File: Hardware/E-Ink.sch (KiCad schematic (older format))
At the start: 34 parts

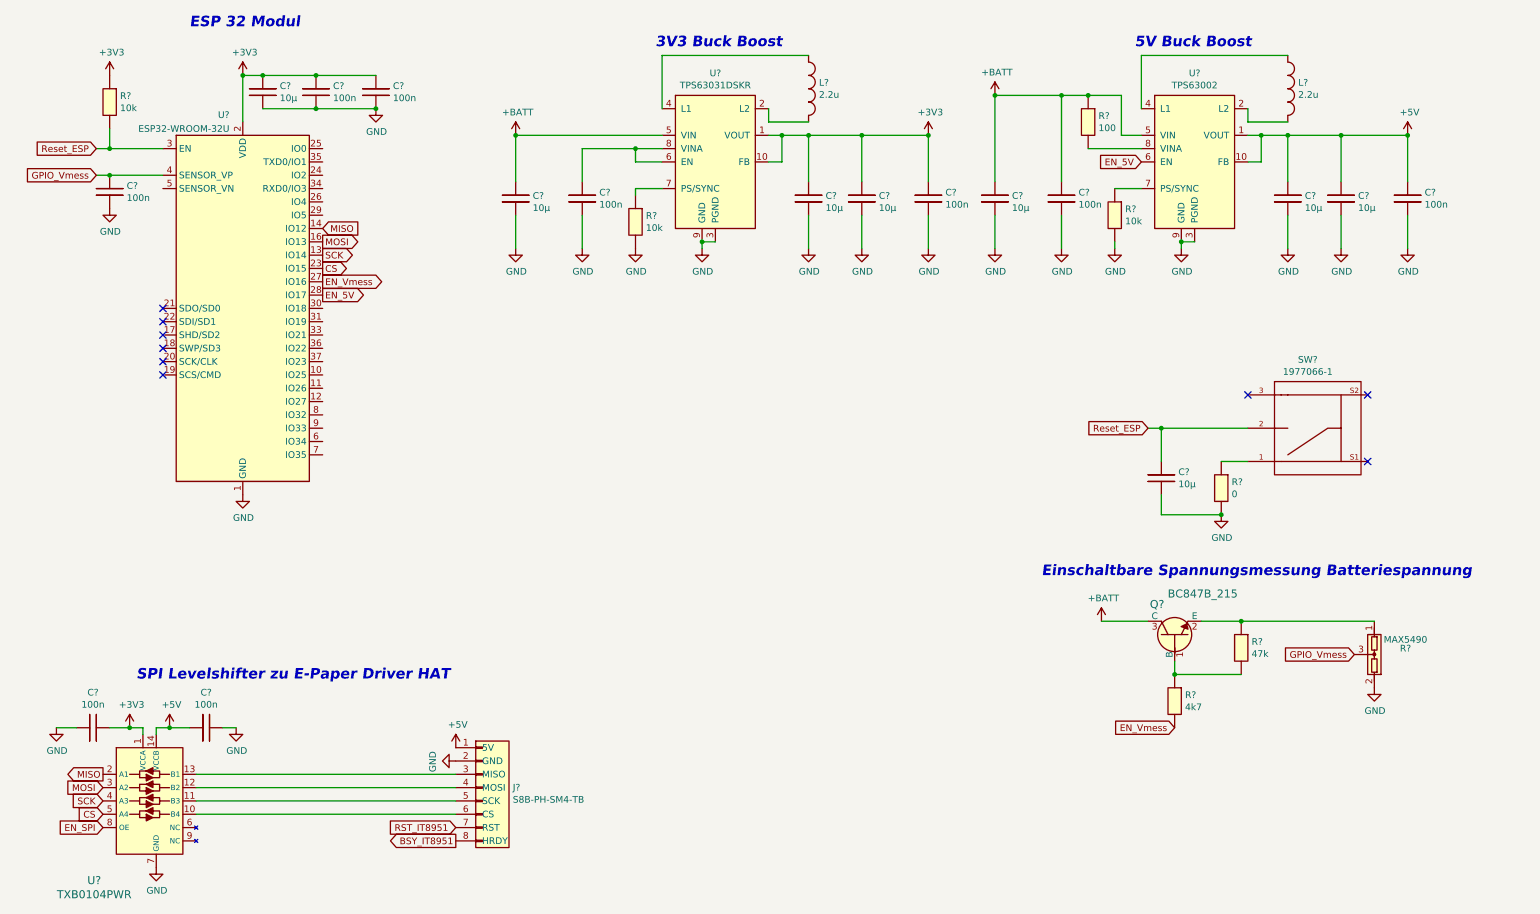
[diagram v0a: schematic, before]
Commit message: Save work at OTH
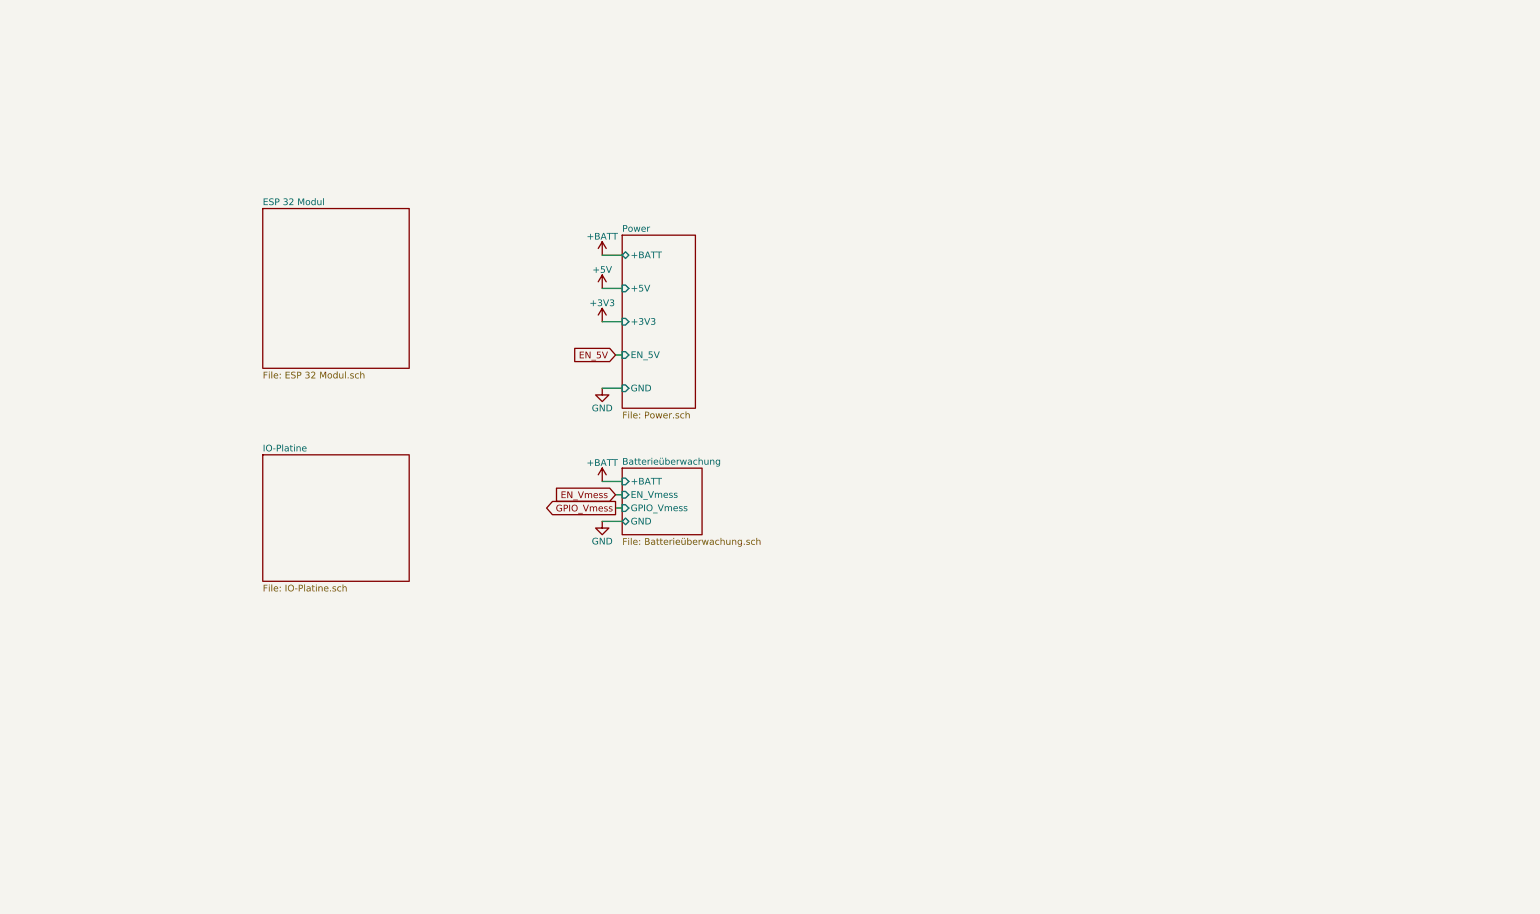
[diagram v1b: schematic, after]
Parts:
- removed C? (x9): 100n, Capacitor_SMD:C_0805_2012Metric_Pad1.15x1.40mm_HandSolder, symbol E-Ink:100n
- removed C? (x8): 10µ, Capacitor_SMD:C_0805_2012Metric_Pad1.15x1.40mm_HandSolder, symbol E-Ink:10µ
- removed J?: S8B-PH-SM4-TB, symbol E-Ink:S8B-PH-SM4-TB
- removed L? (x2): 2.2u, symbol E-Ink:2.2u
- removed Q?: BC847B_215, digikey-footprints:SOT-23-3, symbol dk_Transistors-Bipolar-BJT-Single:BC847B_215
- removed R?: MAX5490, Package_TO_SOT_SMD:SOT-23, symbol E-Ink:MAX5490
- removed R?: 47k, Resistor_SMD:R_0805_2012Metric_Pad1.15x1.40mm_HandSolder, symbol E-Ink:47k
- removed R?: 4k7, Resistor_SMD:R_0805_2012Metric_Pad1.15x1.40mm_HandSolder, symbol E-Ink:4k7
- removed R? (x3): 10k, Resistor_SMD:R_0805_2012Metric_Pad1.15x1.40mm_HandSolder, symbol E-Ink:10k
- removed R?: 100, Resistor_SMD:R_0805_2012Metric_Pad1.15x1.40mm_HandSolder, symbol E-Ink:100
- removed R?: 0, Resistor_SMD:R_0805_2012Metric_Pad1.15x1.40mm_HandSolder, symbol E-Ink:0
- removed SW?: 1977066-1, TE_1977066-1, symbol Pavel_privat:1977066-1
- removed U?: ESP32-WROOM-32U, RF_Module:ESP32-WROOM-32U, symbol E-Ink:ESP32-WROOM-32U
- removed U?: TXB0104PWR, digikey-footprints:TSSOP-14_W4.4mm, symbol E-Ink:TXB0104PWR
- removed U?: TPS63031DSKR, Package_SON:Texas_S-PWSON-N10, symbol E-Ink:TPS63031DSKR
- removed U?: TPS63002, Package_SON:Texas_DRC0010J_ThermalVias, symbol E-Ink:TPS63002DRCR
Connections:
- no-connect marks 9 -> 0
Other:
- note removed: "3V3 Buck Boost"
- note removed: "5V Buck Boost"
- note removed: "ESP 32 Modul\n"
- note removed: "Einschaltbare Spannungsmessung Batteriespannung\n\n"
- note removed: "SPI Levelshifter zu E-Paper Driver HAT\n"

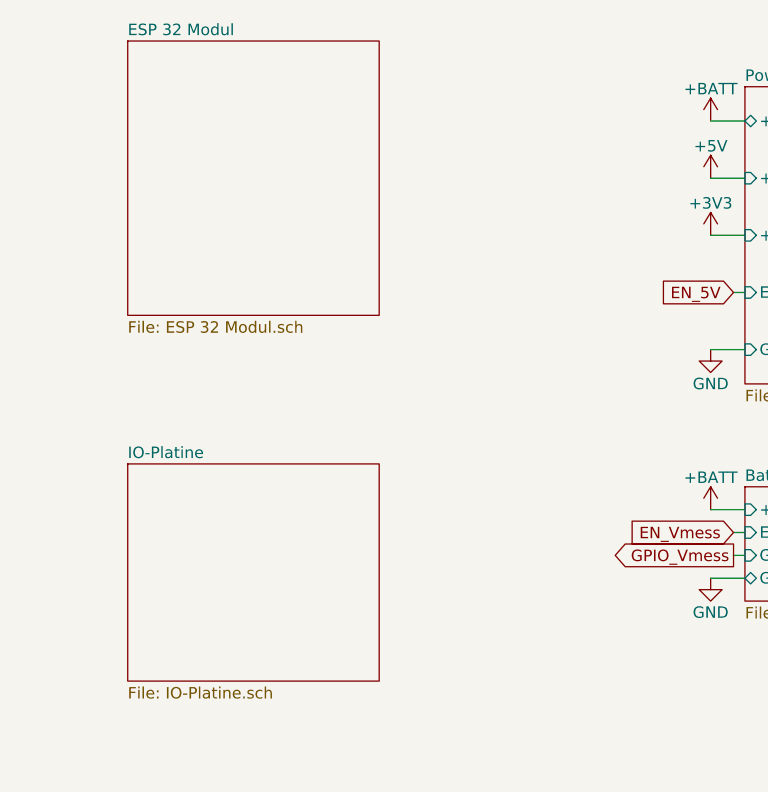
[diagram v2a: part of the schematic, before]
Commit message: Save work from OTH
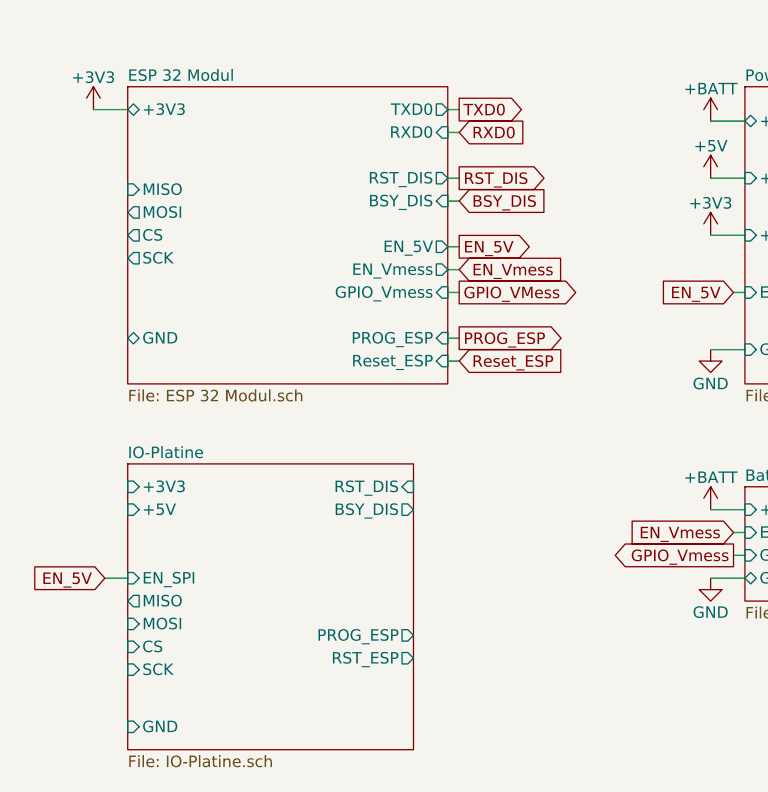
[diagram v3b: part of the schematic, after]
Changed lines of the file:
@@
 EESchema Schematic File Version 4
-EELAYER 30 0
+LIBS:E-Ink-cache
+EELAYER 29 0
 EELAYER END
 $Descr A4 11693 8268
@@
 	4900 4550 4950 4550
 $Sheet
-S 2250 2300 1100 1200
+S 2250 2500 1400 1300
 U 5DE5A7F7
 F0 "ESP 32 Modul" 50
 F1 "ESP 32 Modul.sch" 50
-$EndSheet
-$Sheet
-S 2250 4150 1100 950
-U 5DE7403E
-F0 "IO-Platine" 50
-F1 "IO-Platine.sch" 50
+F2 "Reset_ESP" I R 3650 3700 50
+F3 "GPIO_Vmess" I R 3650 3400 50
+F4 "GND" B L 2250 3600 50
+F5 "+3V3" B L 2250 2600 50
+F6 "TXD0" O R 3650 2600 50
+F7 "MISO" I L 2250 2950 50
+F8 "RXD0" I R 3650 2700 50
+F9 "EN_5V" O R 3650 3200 50
+F10 "EN_Vmess" O R 3650 3300 50
+F11 "CS" O L 2250 3150 50
+F12 "SCK" O L 2250 3250 50
+F13 "MOSI" O L 2250 3050 50
+F14 "PROG_ESP" I R 3650 3600 50
+F15 "RST_DIS" O R 3650 2900 50
+F16 "BSY_DIS" I R 3650 3000 50
 $EndSheet
 $Comp
@@
 Wire Wire Line
 	4800 4650 4950 4650
+$Sheet
+S 2250 4150 1250 1250
+U 5DE7403E
+F0 "IO-Platine" 50
+F1 "IO-Platine.sch" 50
+F2 "EN_SPI" I L 2250 4650 50
+F3 "CS" I L 2250 4950 50
+F4 "SCK" I L 2250 5050 50
+F5 "MOSI" I L 2250 4850 50
+F6 "MISO" O L 2250 4750 50
+F7 "RST_ESP" O R 3500 5000 50
+F8 "+3V3" I L 2250 4250 50
+F9 "+5V" I L 2250 4350 50
+F10 "GND" I L 2250 5300 50
+F11 "RST_DIS" I R 3500 4250 50
+F12 "BSY_DIS" O R 3500 4350 50
+F13 "PROG_ESP" O R 3500 4900 50
+$EndSheet
+$Comp
+L power:+3V3 #PWR?
+U 1 1 5DE68EE7
+P 2100 2600
+F 0 "#PWR?" H 2100 2450 50  0001 C CNN
+F 1 "+3V3" H 2100 2740 50  0000 C CNN
+F 2 "" H 2100 2600 50  0001 C CNN
+F 3 "" H 2100 2600 50  0001 C CNN
+	1    2100 2600
+	1    0    0    -1
+$EndComp
+Wire Wire Line
+	2100 2600 2250 2600
+Text GLabel 3700 2600 2    50   Output ~ 0
+TXD0
+Text GLabel 3700 2700 2    50   Input ~ 0
+RXD0
+Wire Wire Line
+	3700 2600 3650 2600
+Wire Wire Line
+	3650 2700 3700 2700
+Text GLabel 3700 2900 2    50   Output ~ 0
+RST_DIS
+Text GLabel 3700 3000 2    50   Input ~ 0
+BSY_DIS
+Wire Wire Line
+	3700 2900 3650 2900
+Wire Wire Line
+	3650 3000 3700 3000
+Text GLabel 3700 3200 2    50   Output ~ 0
+EN_5V
+Text GLabel 3700 3300 2    50   Input ~ 0
+EN_Vmess
+Wire Wire Line
+	3700 3200 3650 3200
+Wire Wire Line
+	3650 3300 3700 3300
+Text GLabel 3700 3400 2    50   Output ~ 0
+GPIO_VMess
+Wire Wire Line
+	3700 3400 3650 3400
+Text GLabel 3700 3600 2    50   Output ~ 0
+PROG_ESP
+Text GLabel 3700 3700 2    50   Input ~ 0
+Reset_ESP
+Wire Wire Line
+	3700 3600 3650 3600
+Wire Wire Line
+	3650 3700 3700 3700
+Text GLabel 2150 4650 0    50   Input ~ 0
+EN_5V
+Wire Wire Line
+	2150 4650 2250 4650
 $EndSCHEMATC
